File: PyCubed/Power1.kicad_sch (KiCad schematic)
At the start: 38 parts, among them IC1 MAX1771ESA+, J3 1985807, Q1 IRLML2803, Q10 IRLML2803, Q14 MBT2222ADW1T1, Q22 NDS8434, Q23 MBT2222ADW1T1, Q24 SQS141ELNW-T1_GE3, Q25 2SC4713KT146R, Q26 2SC4713KT146R, Q9 IRFR320TRPBF-BE3, U4 ADM1176-1ARMZ-R7

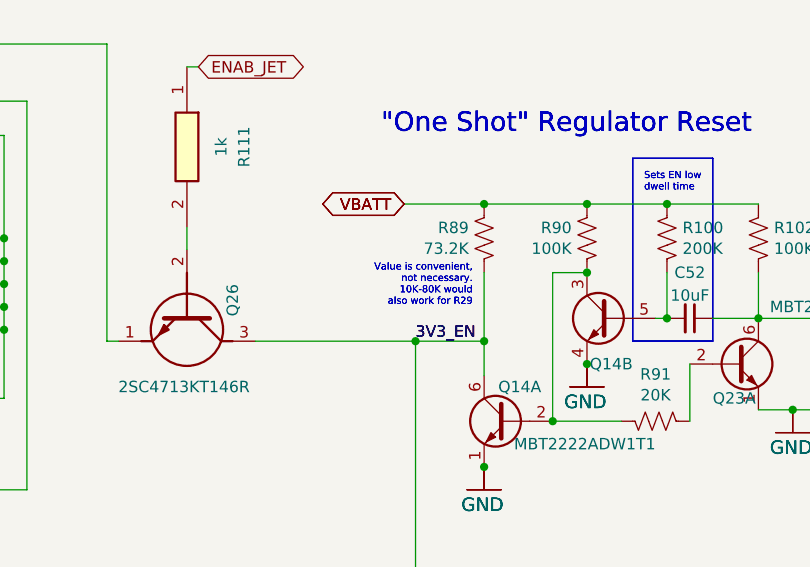
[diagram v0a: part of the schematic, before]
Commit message: PyCubed Schematic Finalized
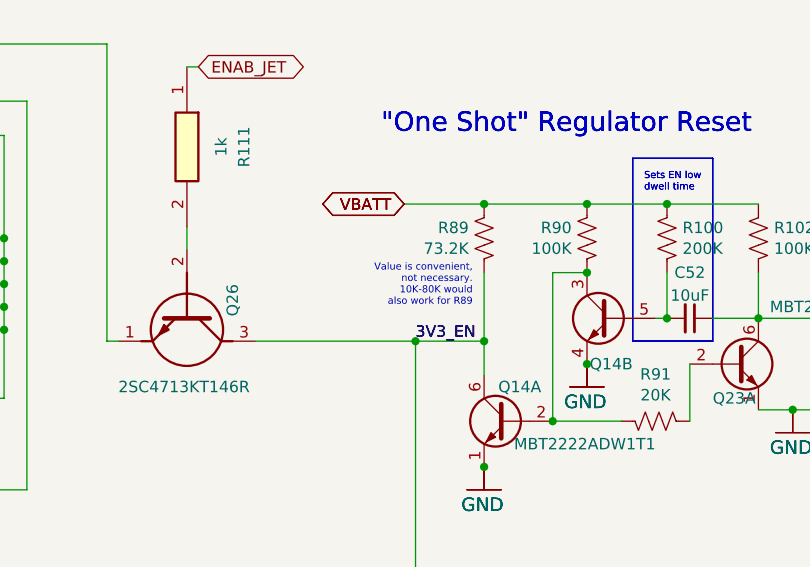
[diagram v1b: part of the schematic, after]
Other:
- note added: "Value is convenient, not necessary. 10K-80K would also work for R89"
- note removed: "Value is convenient, not necessary. 10K-80K would also work for R29"
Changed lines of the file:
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@@
     (effects (font (size 0.7874 0.7874)) (justify left bottom))
   )
-  (text "Value is convenient,\nnot necessary. \n10K-80K would\nalso work for R29"
+  (text "Value is convenient,\nnot necessary. \n10K-80K would\nalso work for R89"
     (at 137.16 46.99 0)
     (effects (font (size 0.7874 0.7874)) (justify right bottom))
-  )
-  (text "Value is convenient,\nnot necessary. \n10K-80K would\nalso work for R29"
-    (at 137.16 46.99 0)
-    (effects (font (size 0.7874 0.7874)) (justify right bottom))
